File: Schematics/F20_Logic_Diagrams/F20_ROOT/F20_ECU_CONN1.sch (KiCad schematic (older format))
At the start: 1 part

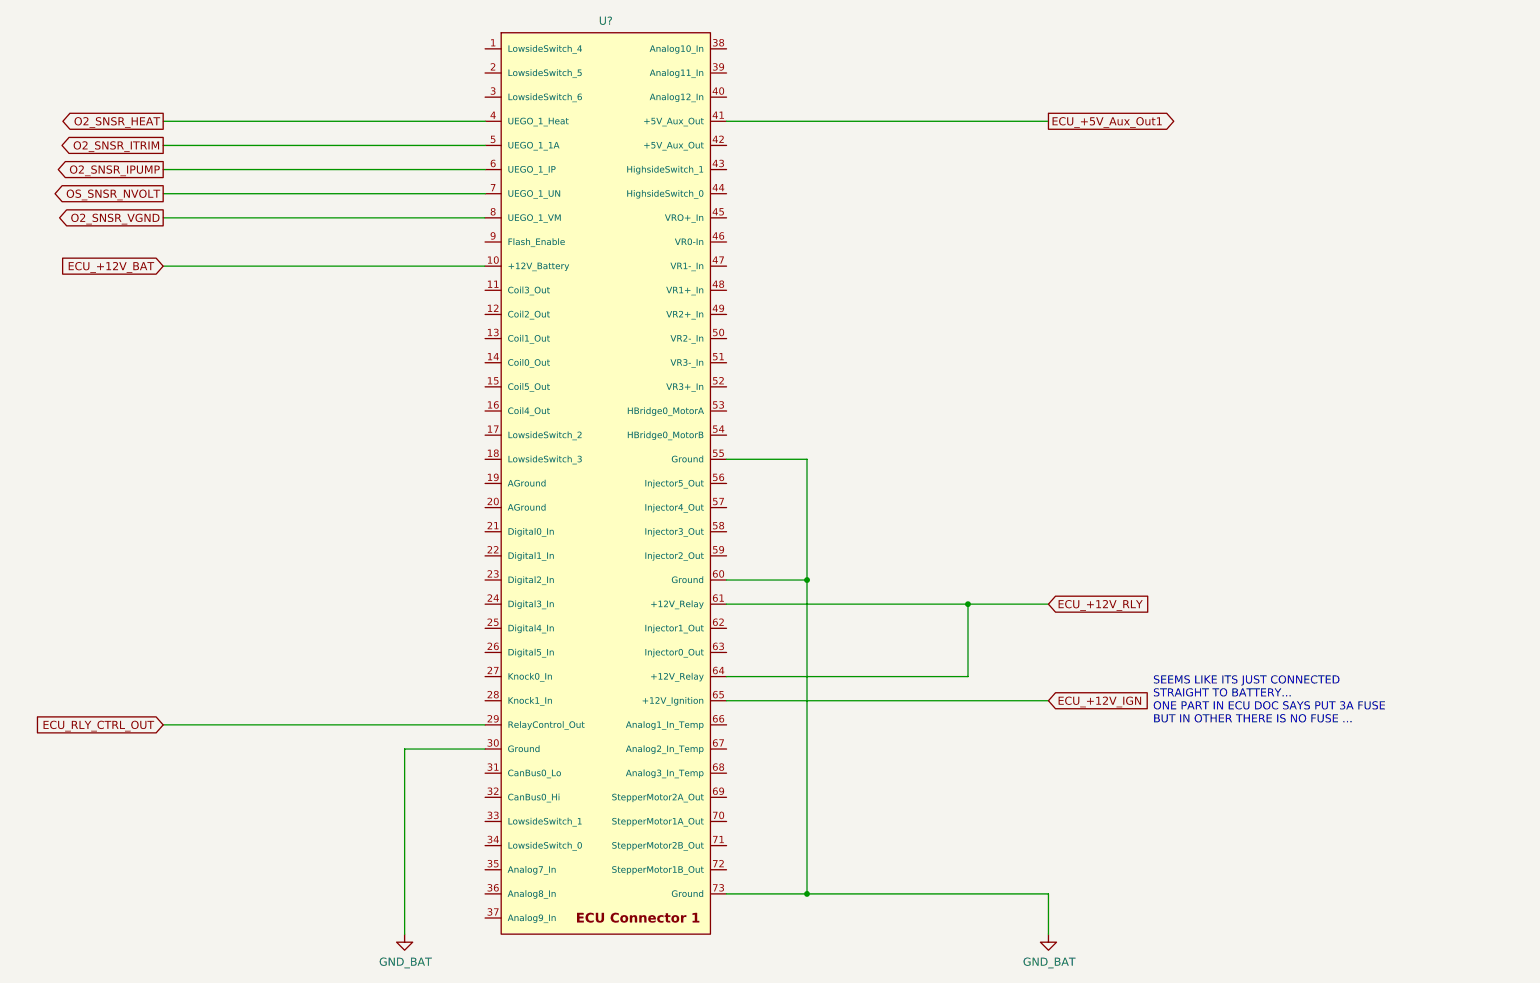
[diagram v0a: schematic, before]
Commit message: 02/18/20 update
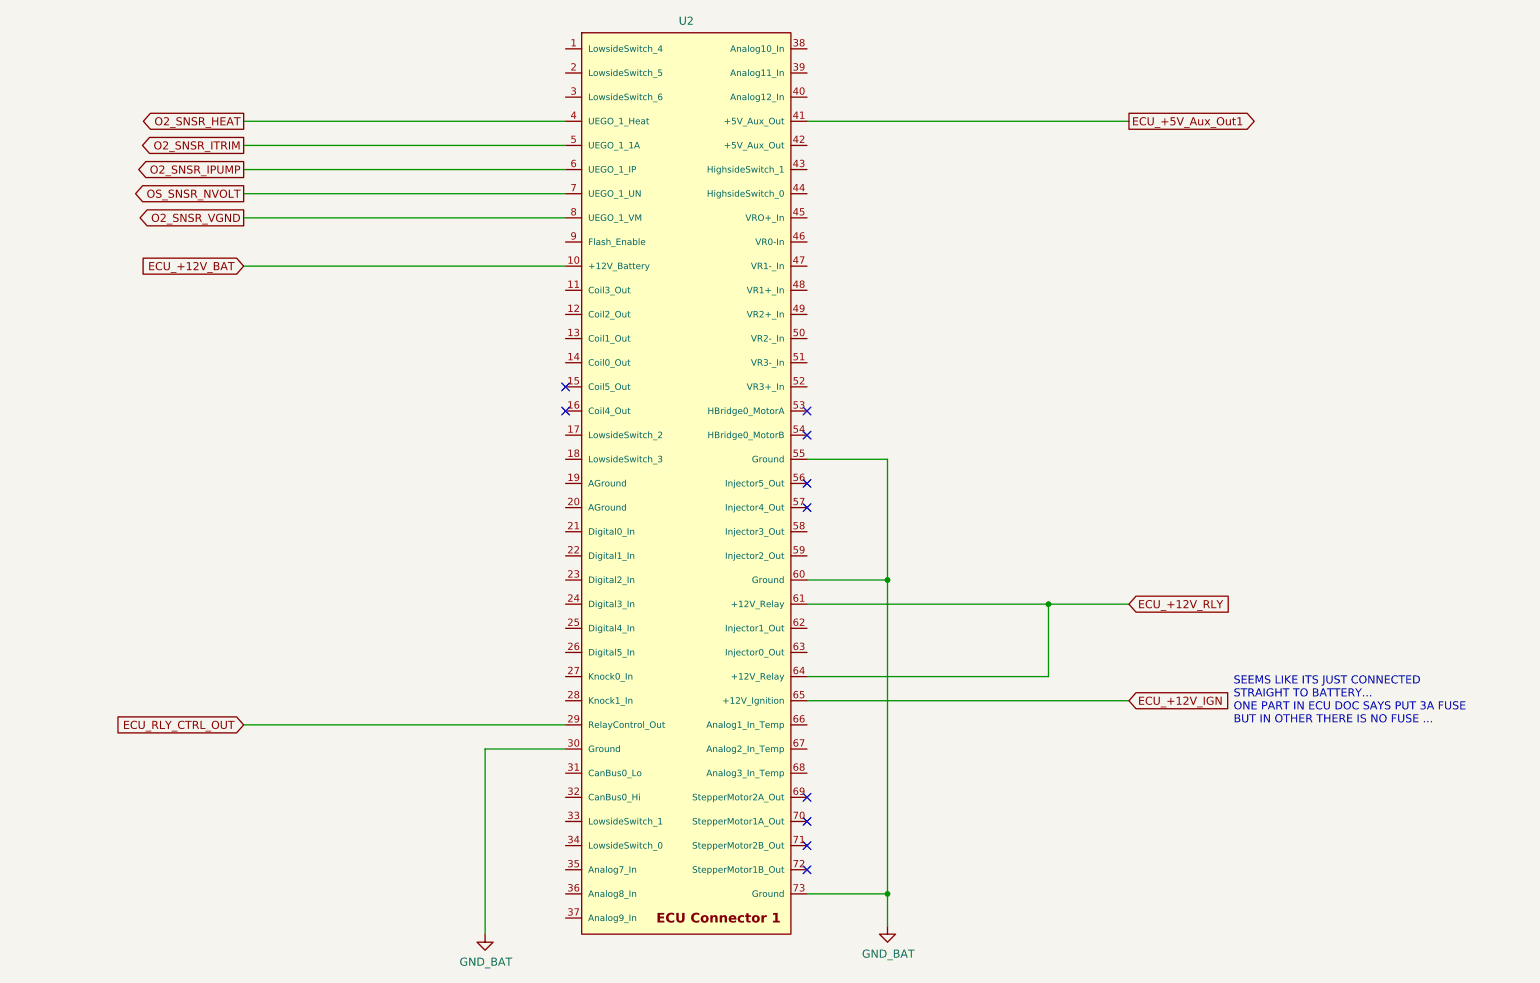
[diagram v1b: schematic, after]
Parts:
- gave numbers to parts that had none: 1
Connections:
- no-connect marks 0 -> 10
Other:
- moved on the sheet: U2
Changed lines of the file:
@@
 $Descr A 11000 8500
 encoding utf-8
-Sheet 3 11
+Sheet 3 13
 Title "ECU Connector 1"
 Date ""
@@
 $EndDescr
 $Comp
-L FSAE_Library:ECU_Conn1 U?
+L FSAE_Library:ECU_Conn1 U2
 U 1 1 5E3C649A
-P 4000 1000
-F 0 "U?" H 4750 1173 50  0000 C CNN
-F 1 "ECU_Conn1" H 4750 1150 50  0001 C CNN
-F 2 "" H 4500 2000 50  0001 C CNN
-F 3 "" H 4500 2000 50  0001 C CNN
-F 4 "https://www.molex.com/molex/products/part-detail/pcb_headers/0313872034" H 3950 1400 50  0001 C CNN "Header Datasheet"
-F 5 "https://www.molex.com/molex/products/part-detail/crimp_housings/0345660203" H 4000 1500 50  0001 C CNN "Plug Datasheet"
-	1    4000 1000
+P 4500 1000
+F 0 "U2" H 5250 1173 50  0000 C CNN
+F 1 "ECU_Conn1" H 5250 1150 50  0001 C CNN
+F 2 "" H 5000 2000 50  0001 C CNN
+F 3 "" H 5000 2000 50  0001 C CNN
+F 4 "https://www.molex.com/molex/products/part-detail/pcb_headers/0313872034" H 4450 1400 50  0001 C CNN "Header Datasheet"
+F 5 "https://www.molex.com/molex/products/part-detail/crimp_housings/0345660203" H 4500 1500 50  0001 C CNN "Plug Datasheet"
+	1    4500 1000
 	1    0    0    -1
 $EndComp
-Text GLabel 7500 1450 2    50   Output ~ 0
+Text GLabel 8000 1450 2    50   Output ~ 0
 ECU_+5V_Aux_Out1
-Text GLabel 2000 1450 0    50   Output ~ 0
+Text GLabel 2500 1450 0    50   Output ~ 0
 O2_SNSR_HEAT
-Text GLabel 2000 1900 0    50   Output ~ 0
+Text GLabel 2500 1900 0    50   Output ~ 0
 OS_SNSR_NVOLT
-Text GLabel 2000 1750 0    50   Output ~ 0
+Text GLabel 2500 1750 0    50   Output ~ 0
 O2_SNSR_IPUMP
-Text GLabel 2000 2050 0    50   Output ~ 0
+Text GLabel 2500 2050 0    50   Output ~ 0
 O2_SNSR_VGND
-Text GLabel 2000 1600 0    50   Output ~ 0
+Text GLabel 2500 1600 0    50   Output ~ 0
 O2_SNSR_ITRIM
 Wire Wire Line
-	2000 1450 4000 1450
+	2500 1450 4500 1450
 Wire Wire Line
-	4000 1600 2000 1600
+	4500 1600 2500 1600
 Wire Wire Line
-	2000 1750 4000 1750
+	2500 1750 4500 1750
 Wire Wire Line
-	4000 1900 2000 1900
+	4500 1900 2500 1900
 Wire Wire Line
-	2000 2050 4000 2050
+	2500 2050 4500 2050
 Wire Wire Line
-	7500 1450 5500 1450
+	8000 1450 6000 1450
 Wire Wire Line
-	5500 4450 7000 4450
+	6000 4450 7500 4450
 Wire Wire Line
-	5500 4900 7000 4900
+	6000 4900 7500 4900
 Wire Wire Line
-	7000 4900 7000 4450
-Connection ~ 7000 4450
+	7500 4900 7500 4450
+Connection ~ 7500 4450
 Wire Wire Line
-	7000 4450 7500 4450
-Text GLabel 7500 4450 2    50   Input ~ 0
+	7500 4450 8000 4450
+Text GLabel 8000 4450 2    50   Input ~ 0
 ECU_+12V_RLY
-Text GLabel 2000 5200 0    50   Input ~ 0
+Text GLabel 2500 5200 0    50   Input ~ 0
 ECU_RLY_CTRL_OUT
 Wire Wire Line
-	2000 5200 4000 5200
+	2500 5200 4500 5200
 $Comp
-L FSAE_Library:GND_BAT #PWR?
+L FSAE_Library:GND_BAT #PWR02
 U 1 1 5E44A710
-P 7500 6500
-F 0 "#PWR?" H 7500 6250 50  0001 C CNN
-F 1 "GND_BAT" H 7505 6327 50  0000 C CNN
-F 2 "" H 7500 6500 50  0001 C CNN
-F 3 "" H 7500 6500 50  0001 C CNN
-	1    7500 6500
+P 6500 6450
+F 0 "#PWR02" H 6500 6200 50  0001 C CNN
+F 1 "GND_BAT" H 6505 6277 50  0000 C CNN
+F 2 "" H 6500 6450 50  0001 C CNN
+F 3 "" H 6500 6450 50  0001 C CNN
+	1    6500 6450
 	1    0    0    -1
 $EndComp
 Wire Wire Line
-	7500 6500 7500 6250
+	6500 6450 6500 6250
 Wire Wire Line
-	7500 6250 6000 6250
+	6000 3550 6500 3550
 Wire Wire Line
-	5500 3550 6000 3550
+	6500 3550 6500 4300
+Connection ~ 6500 6250
 Wire Wire Line
-	6000 3550 6000 4300
-Connection ~ 6000 6250
+	6500 6250 6000 6250
 Wire Wire Line
-	6000 6250 5500 6250
+	6000 4300 6500 4300
+Connection ~ 6500 4300
 Wire Wire Line
-	5500 4300 6000 4300
-Connection ~ 6000 4300
+	4500 5350 4000 5350
 Wire Wire Line
-	6000 4300 6000 6250
-Wire Wire Line
-	4000 5350 3500 5350
-Wire Wire Line
-	3500 5350 3500 6500
+	4000 5350 4000 6500
 $Comp
-L FSAE_Library:GND_BAT #PWR?
+L FSAE_Library:GND_BAT #PWR03
 U 1 1 5E4538FC
-P 3500 6500
-F 0 "#PWR?" H 3500 6250 50  0001 C CNN
-F 1 "GND_BAT" H 3505 6327 50  0000 C CNN
-F 2 "" H 3500 6500 50  0001 C CNN
-F 3 "" H 3500 6500 50  0001 C CNN
-	1    3500 6500
+P 4000 6500
+F 0 "#PWR03" H 4000 6250 50  0001 C CNN
+F 1 "GND_BAT" H 4005 6327 50  0000 C CNN
+F 2 "" H 4000 6500 50  0001 C CNN
+F 3 "" H 4000 6500 50  0001 C CNN
+	1    4000 6500
 	1    0    0    -1
 $EndComp
-Text GLabel 2000 2350 0    50   Input ~ 0
+Text GLabel 2500 2350 0    50   Input ~ 0
 ECU_+12V_BAT
 Wire Wire Line
-	2000 2350 4000 2350
+	2500 2350 4500 2350
 Wire Wire Line
-	5500 5050 7500 5050
-Text Notes 8150 5200 0    50   ~ 0
+	6000 5050 8000 5050
+Text Notes 8650 5200 0    50   ~ 0
 SEEMS LIKE ITS JUST CONNECTED\nSTRAIGHT TO BATTERY...\nONE PART IN ECU DOC SAYS PUT 3A FUSE\nBUT IN OTHER THERE IS NO FUSE ...
-Text GLabel 7500 5050 2    50   Input ~ 0
+Text GLabel 8000 5050 2    50   Input ~ 0
 ECU_+12V_IGN
+NoConn ~ 6000 6100
+Wire Wire Line
+	6500 4300 6500 6250
+NoConn ~ 6000 5950
+NoConn ~ 6000 5800
+NoConn ~ 6000 5650
+NoConn ~ 6000 3700
+NoConn ~ 6000 3850
+NoConn ~ 6000 3400
+NoConn ~ 6000 3250
+NoConn ~ 4500 3100
+NoConn ~ 4500 3250
 $EndSCHEMATC
